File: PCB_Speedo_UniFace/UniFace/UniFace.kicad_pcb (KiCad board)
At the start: 2 copper layers, 44 x 44 mm, 0 parts

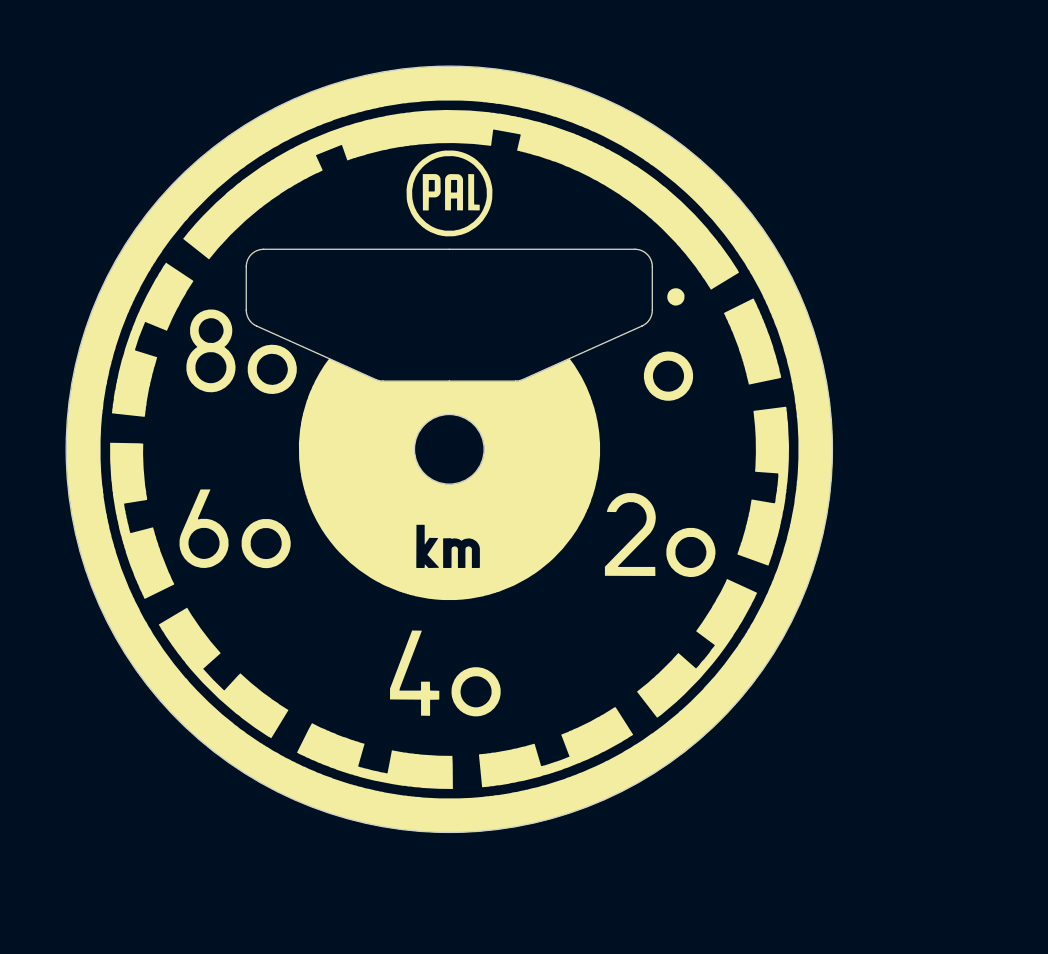
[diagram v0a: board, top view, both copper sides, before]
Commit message: UniFace PCB
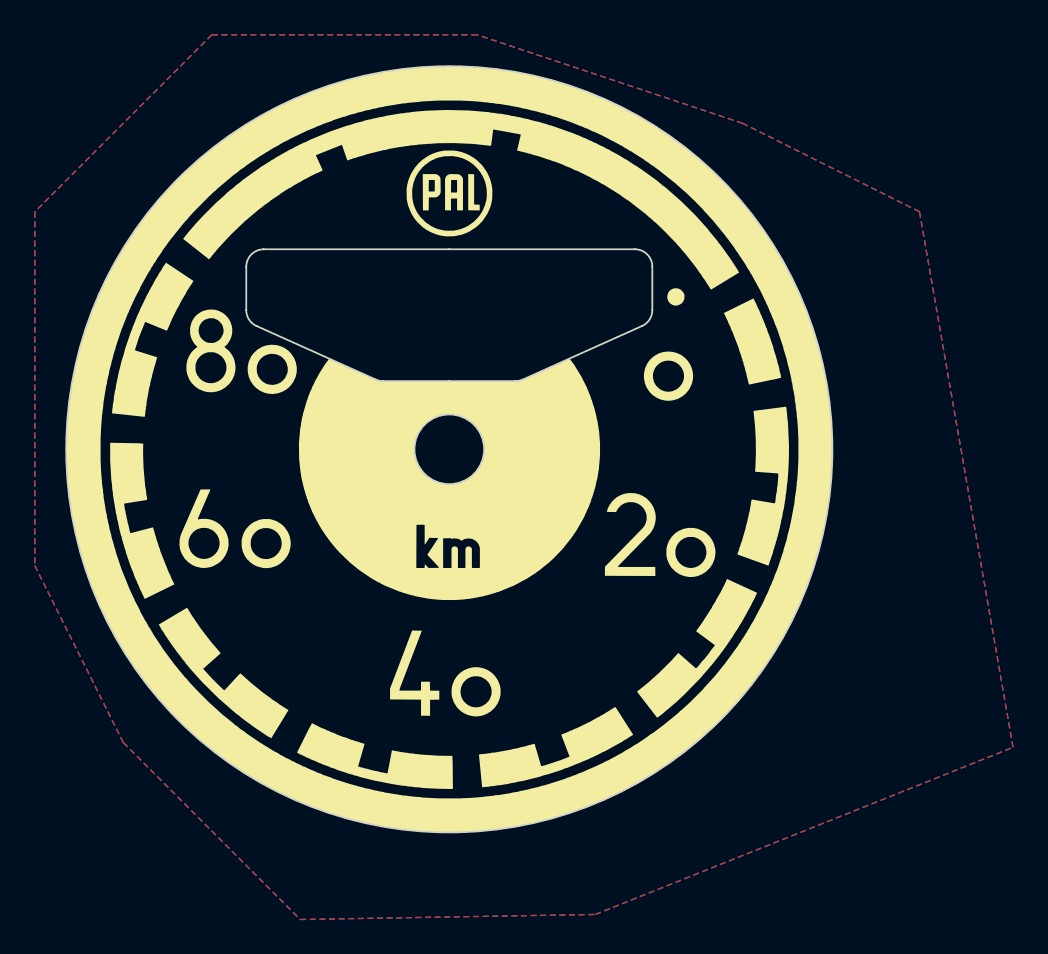
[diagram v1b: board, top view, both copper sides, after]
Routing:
- added copper zone on B.Cu, net GND
- added copper zone on F.Cu, net GND

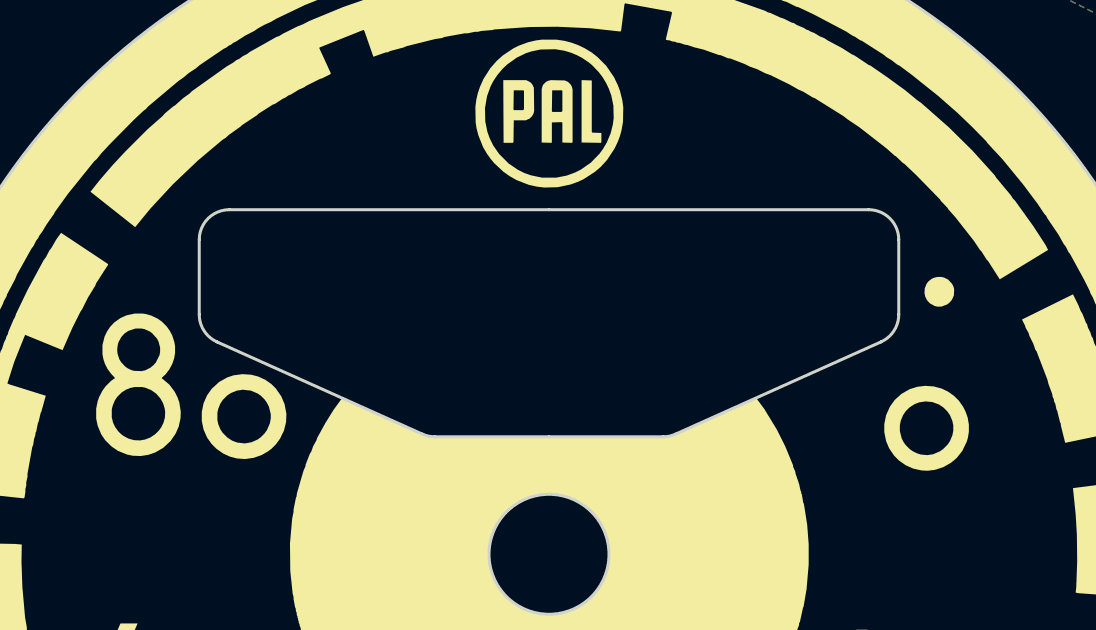
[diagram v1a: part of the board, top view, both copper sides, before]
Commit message: dalsi verze uniface
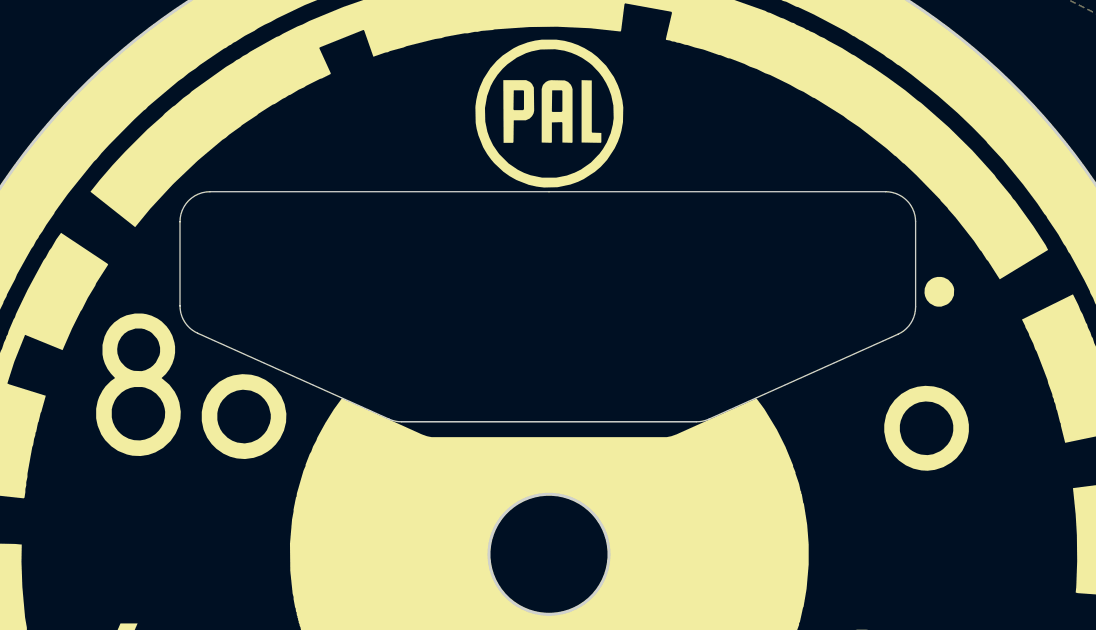
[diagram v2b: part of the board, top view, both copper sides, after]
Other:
- outline, holes or cut-outs redrawn
